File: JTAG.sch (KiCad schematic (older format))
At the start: 27 parts, among them CN5 CONN_RCPT_USB2.0_MINI_B_SMD_R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, U15 FT2232HL-REEL, X2 ABM3B-12.000MHZ

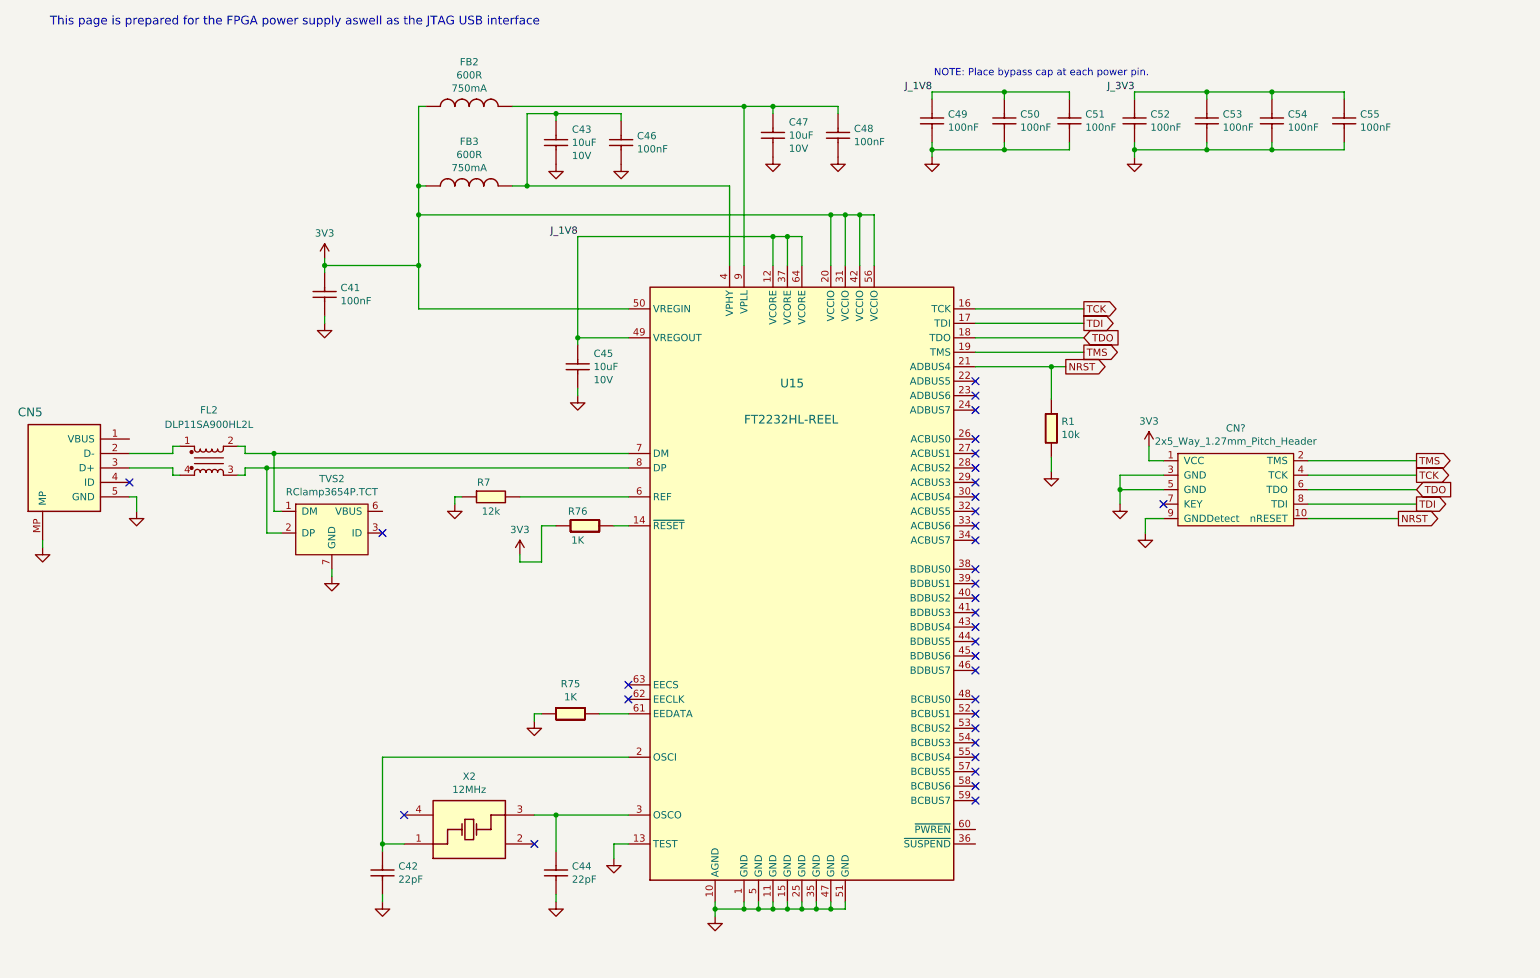
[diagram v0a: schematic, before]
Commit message: Update JTAG.sch
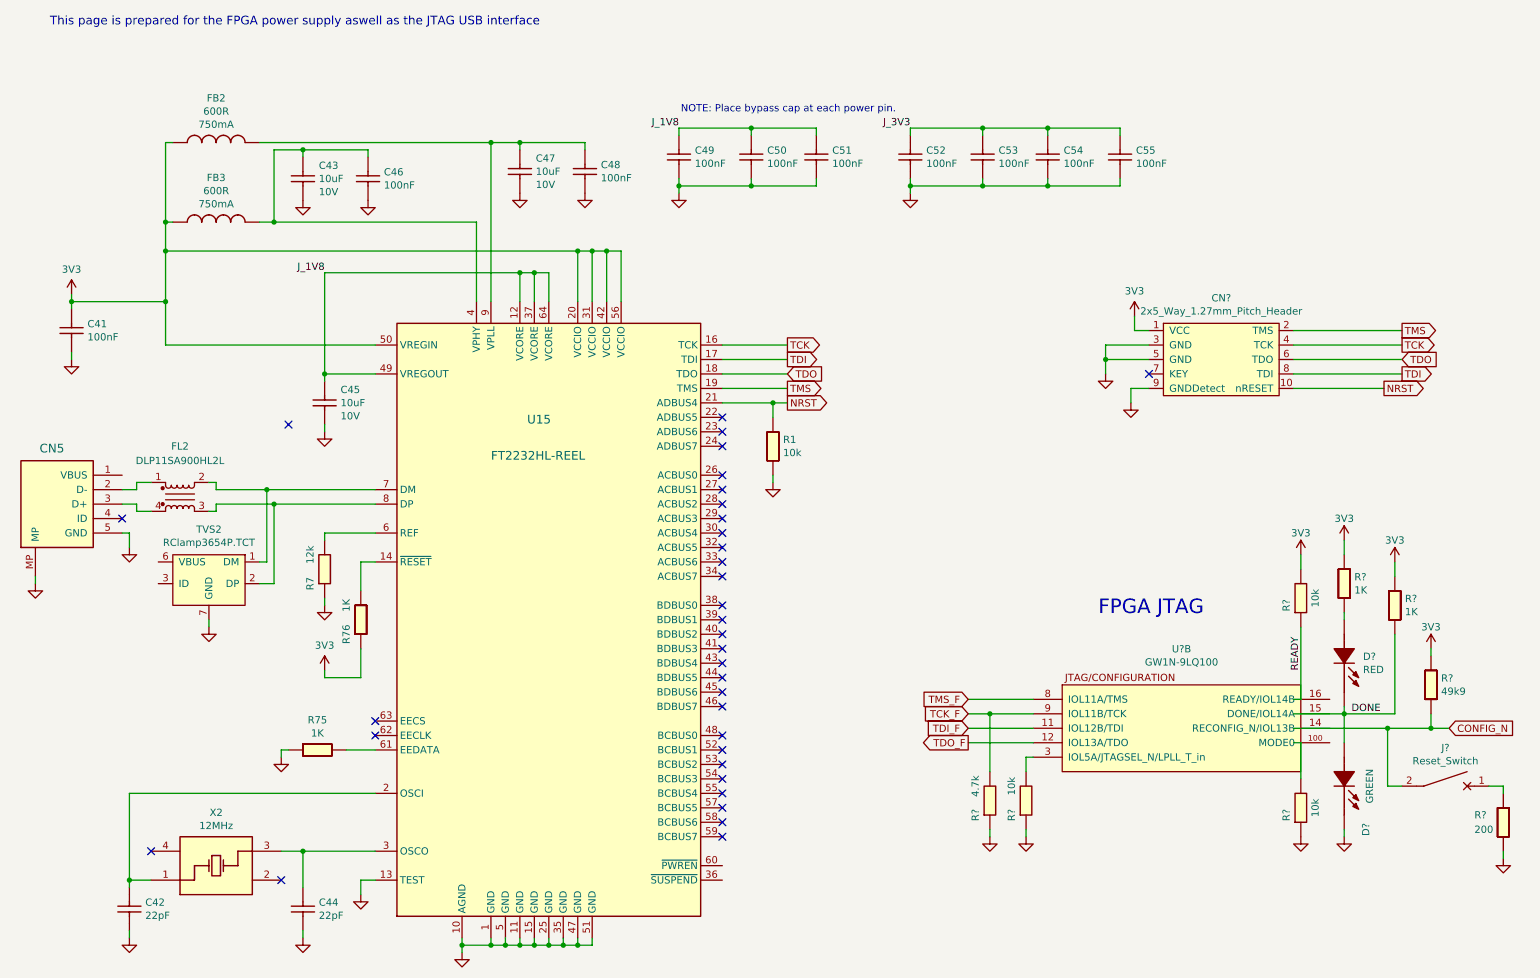
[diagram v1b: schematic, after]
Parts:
- added D?: LED_GREEN_0603_SMD, symbol OpenVent:LED_GREEN_0603_SMD
- added D?: LED_Red_0603_SMD, symbol OpenVent:LED_Red_0603_SMD
- added J?: Reset_Switch, symbol Device:CircuitBreaker_1P
- added R? (x4): 12k_0603_Chip_Resistor,_1%,_0.1W, Resistor_SMD:R_0603_1608Metric, symbol OpenVent:12k_0603_Chip_Resistor,_1%,_0.1W
- added R?: R_0603_200_0.1W_1%, Resistor_SMD:R_0603_1608Metric, symbol OpenVent:R_0603_200_0.1W_1%
- added R? (x2): 1K_0603_Chip_Resistor,_1%,_0.1W, symbol OpenVent:1K_0603_Chip_Resistor,_1%,_0.1W
- added R?: R_0603_49k9_0.1W_1%, symbol OpenVent:R_0603_49k9_0.1W_1%
- added U?: GW1N-9LQ100, symbol OpenVent:GW1N-9LQ100
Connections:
- net +3V3: now also R?.1, R?.1, R?.1, R?.2
- net GND: now also D?.2 (CATHODE), R?.1, R?.1, R?.1, R?.2
- new net: J?.1, R?.1
- new net: D?.1 (ANODE), R?.2
- new net: R?.2, U?.3 (IOL5A/JTAGSEL_N/LPLL_T_in)
- new net CONFIG_N: J?.2, R?.2
- new net DONE: D?.1 (ANODE), D?.2 (CATHODE), R?.2
- new net READY: R?.1
- new net TCK_F: R?.2, U?.9 (IOL11B/TCK)
- new net TDI_F: U?.11 (IOL12B/TDI)
- new net TDO_F: U?.12 (IOL13A/TDO)
- new net TMS_F: U?.8 (IOL11A/TMS)
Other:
- note added: "FPGA JTAG\n"
- moved on the sheet: C41, C42, C43, C44, C45, C46, C47, C48, C49, C50, C51, C52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
